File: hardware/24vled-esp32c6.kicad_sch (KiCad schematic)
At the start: 23 parts, among them J1 2601-1106, J2 Conn_01x02_Pin, Q1 AO3400A, Q2 AO3400A, Q3 AO3400A, Q4 AO3400A, Q5 AO3400A, U1 R-78E5.0-1.0

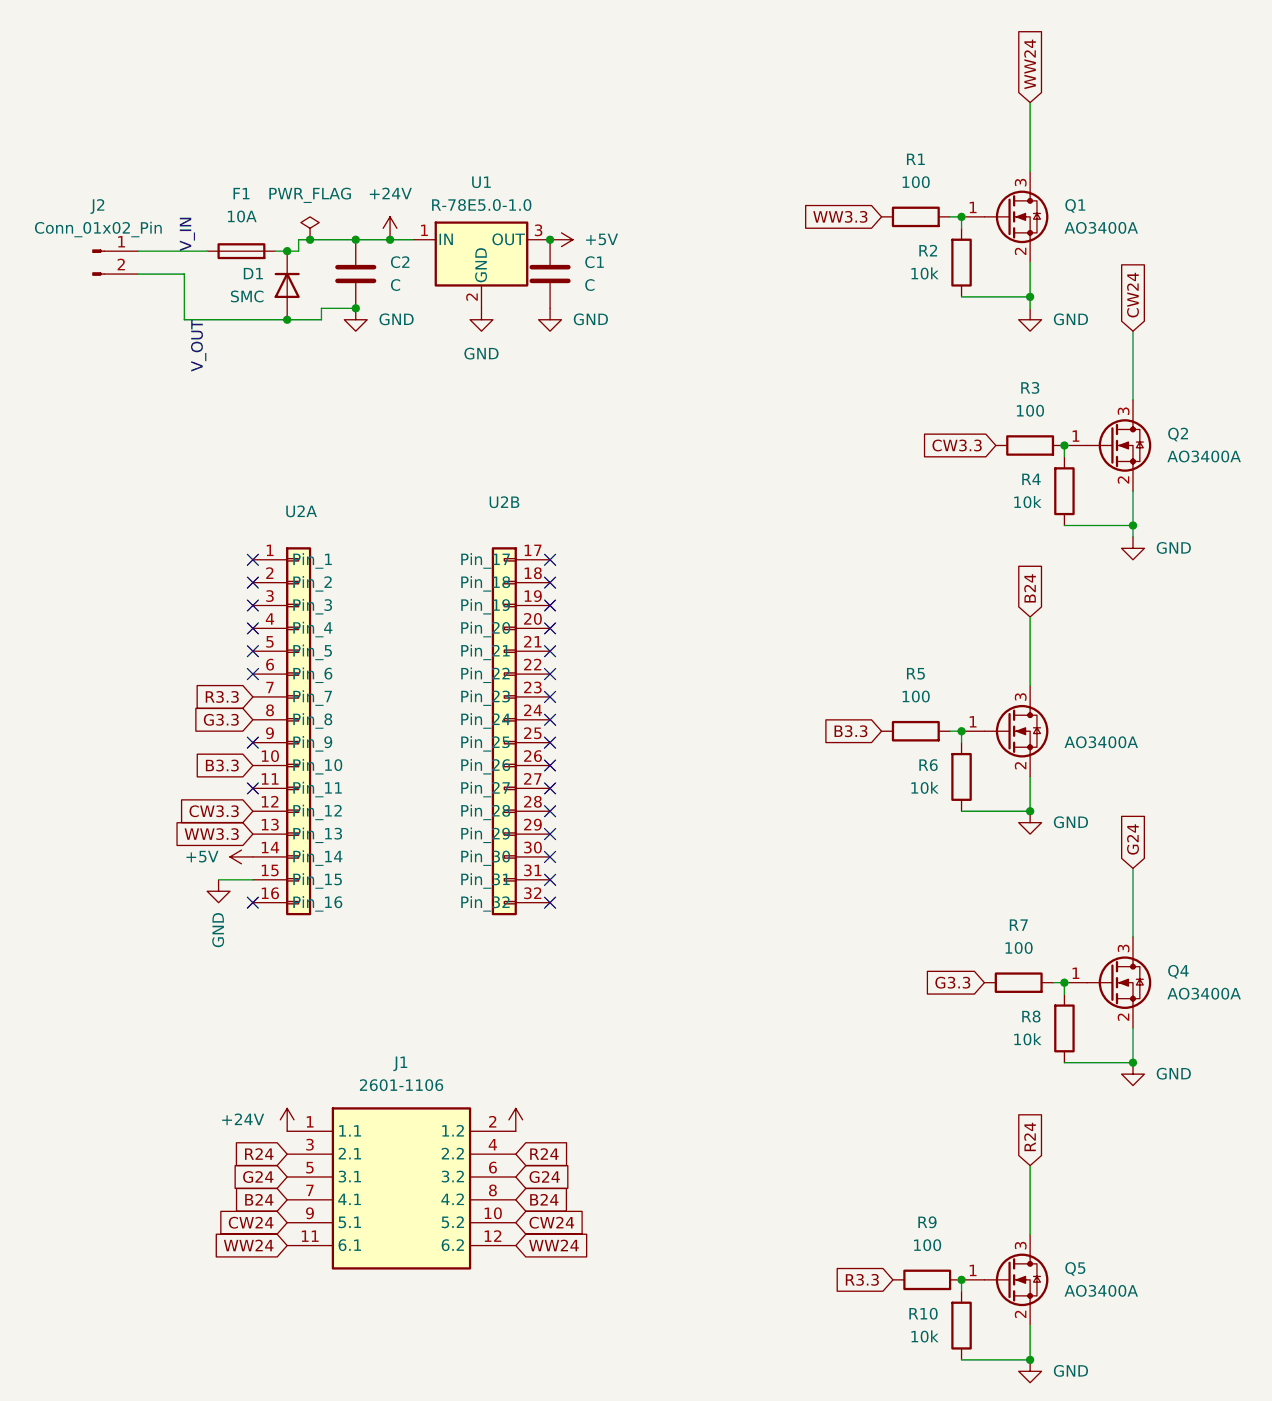
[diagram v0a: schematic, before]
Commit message: final version!
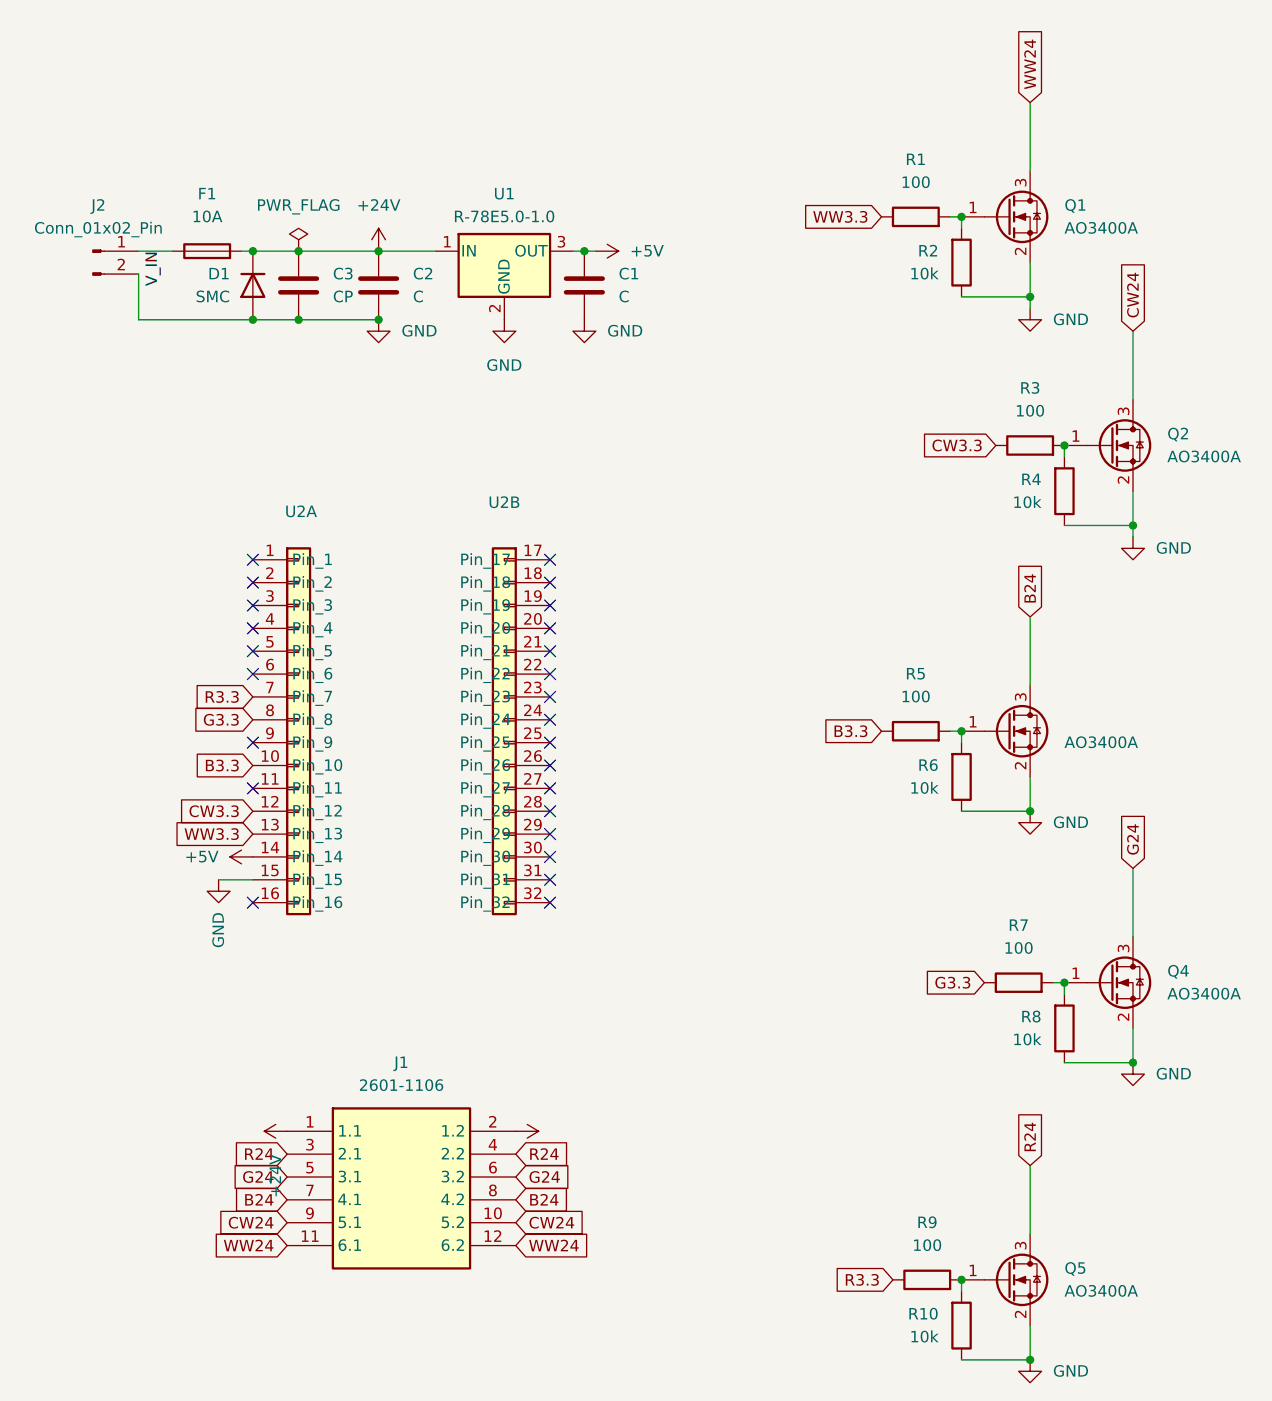
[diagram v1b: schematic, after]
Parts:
- added C3: CP, Capacitor_THT:CP_Radial_D8.0mm_P5.00mm, symbol Device:C
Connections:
- net +24V: now also C3.1
- net GND: now also C3.2
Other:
- moved on the sheet: C1, C2, D1, F1, U1
